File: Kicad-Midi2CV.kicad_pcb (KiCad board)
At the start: 2 copper layers, 99.7 x 99.7 mm, 87 parts, among them IC1 MCP4725module, IC2 MCP4725module, J1 Doepfer connector, J10 CV4, J11 Gate1, J12 GateConn, J13 Gate2, J14 Gate3, J15 Gate4, J16 I2C_Conn, J17 I2C_Conn, J18 GateConn, J19 CV7 in, J2 Vin 7-12v, J20 CV3 in, J3 MIDI OUT, J4 CV6 in, J5 Power Conn, J6 CV1, J7 CV2, J8 MIDI IN, J9 CV3, Q1 MMBT2222A, Q2 MMBT2222A, SW1 KY40_Rotary_Encoder_Module, U1 TL072, U2 EL814, U3 MCP4728

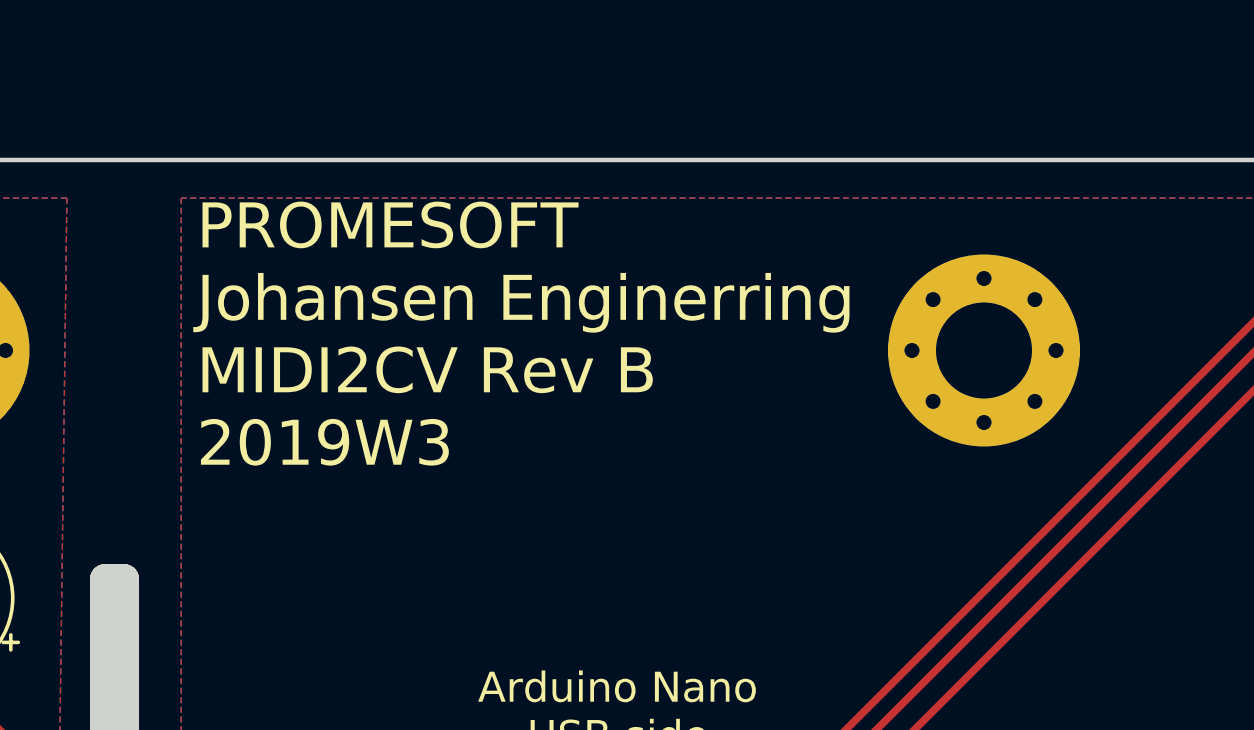
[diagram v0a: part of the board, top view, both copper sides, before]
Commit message: Minor
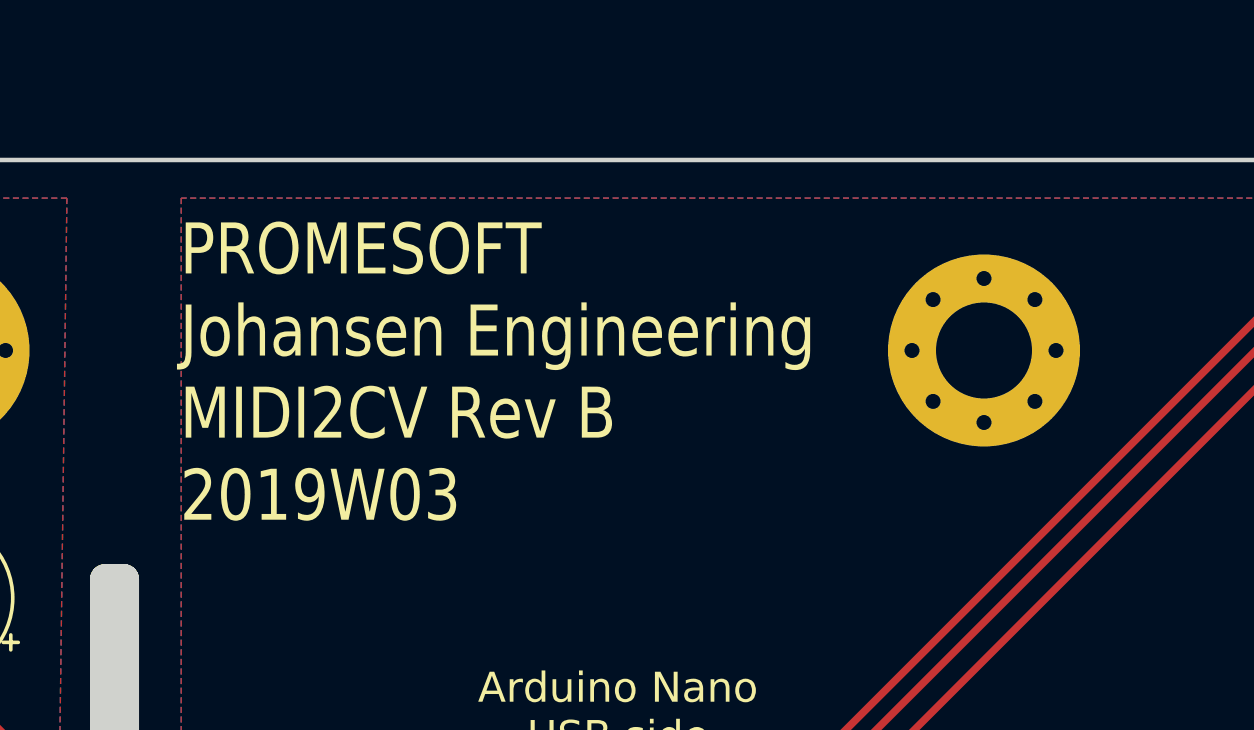
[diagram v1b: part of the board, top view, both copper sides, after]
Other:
- board text added: "PROMESOFT Johansen Engineering MIDI2CV Rev B 2019W03"
- board text removed: "PROMESOFT Johansen Enginerring MIDI2CV Rev B 2019W3"
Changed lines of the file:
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@@
     (effects (font (size 1.5 1.5) (thickness 0.3)) (justify left mirror))
   )
-  (gr_text "PROMESOFT\nJohansen Enginerring\nMIDI2CV Rev B\n2019W3" (at 66.548 31.242) (layer F.SilkS)
-    (effects (font (size 1.5 1.5) (thickness 0.3)) (justify left))
+  (gr_text "PROMESOFT\nJohansen Engineering\nMIDI2CV Rev B\n2019W03" (at 66 32.5) (layer F.SilkS)
+    (effects (font (size 1.7 1.42) (thickness 0.3)) (justify left))
   )
   (gr_line (start 90.2 25.4) (end 90.2 125.095) (layer Dwgs.User) (width 0.15))
@@
   (segment (start 72.898 52.07) (end 67.564 52.07) (width 0.5) (layer F.Cu) (net 2))
   (segment (start 67.564 52.07) (end 66.548 53.086) (width 0.5) (layer F.Cu) (net 2))
-  (via (at 85.852 84.400001) (size 0.8) (drill 0.4) (layers F.Cu B.Cu) (net 59))
-  (segment (start 87.702001 82.55) (end 88.138 82.55) (width 0.25) (layer B.Cu) (net 59))
-  (segment (start 85.852 84.400001) (end 87.702001 82.55) (width 0.25) (layer B.Cu) (net 59))
   (segment (start 72.818764 57.070764) (end 72.898 57.15) (width 0.25) (layer F.Cu) (net 3))
   (segment (start 70.206317 57.070764) (end 72.818764 57.070764) (width 0.25) (layer F.Cu) (net 3))
@@
   (segment (start 88.138 85.09) (end 88.138 86.14) (width 0.25) (layer F.Cu) (net 58))
   (via (at 81 92.4) (size 0.8) (drill 0.4) (layers F.Cu B.Cu) (net 58))
+  (via (at 85.852 84.400001) (size 0.8) (drill 0.4) (layers F.Cu B.Cu) (net 59))
+  (segment (start 87.702001 82.55) (end 88.138 82.55) (width 0.25) (layer B.Cu) (net 59))
+  (segment (start 85.852 84.400001) (end 87.702001 82.55) (width 0.25) (layer B.Cu) (net 59))
   (segment (start 80.042856 92.28414) (end 80.042856 93.386319) (width 0.25) (layer F.Cu) (net 59))
   (segment (start 80.042856 93.386319) (end 80.892855 94.236318) (width 0.25) (layer F.Cu) (net 59))
